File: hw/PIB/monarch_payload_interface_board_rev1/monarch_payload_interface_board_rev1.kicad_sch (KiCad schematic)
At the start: 0 parts

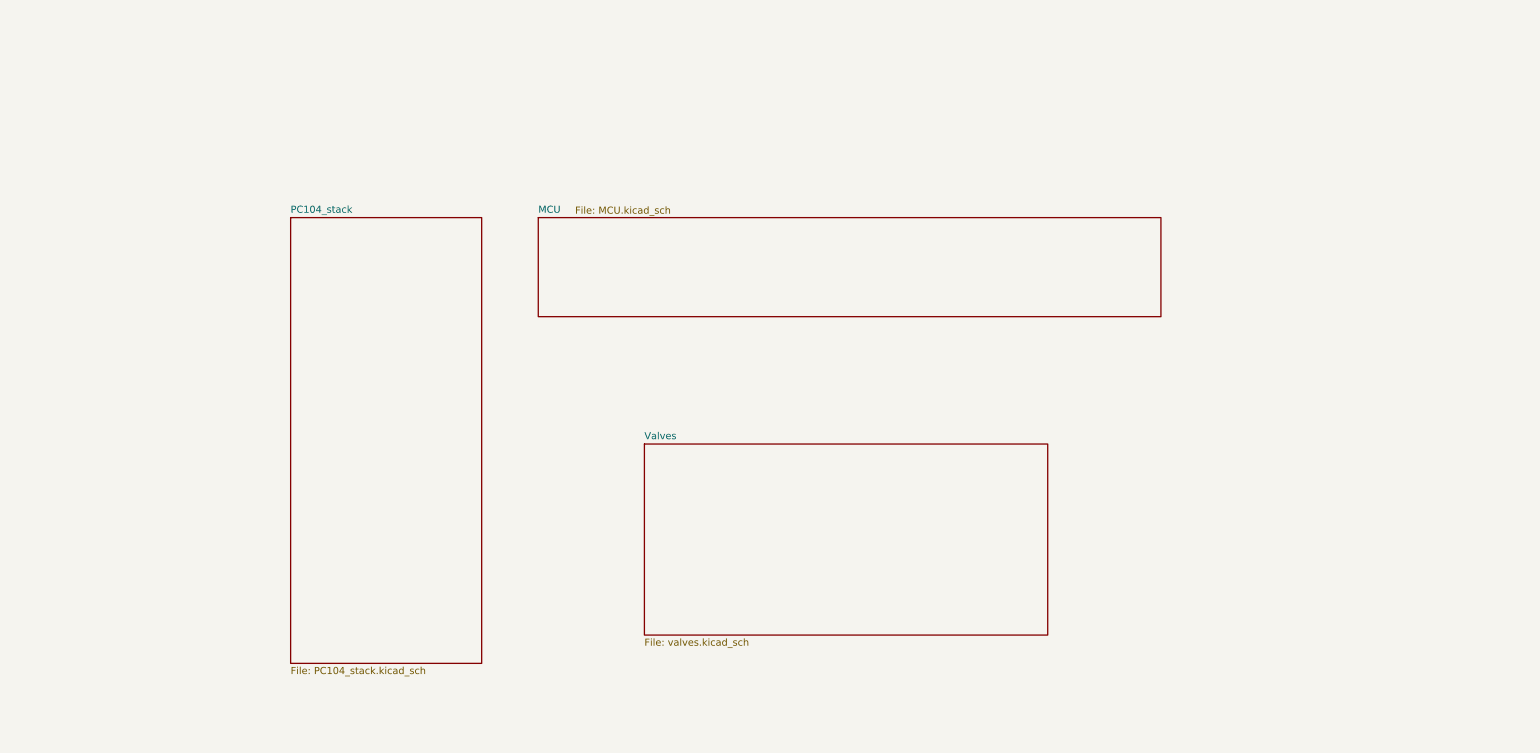
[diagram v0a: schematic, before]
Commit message: More components
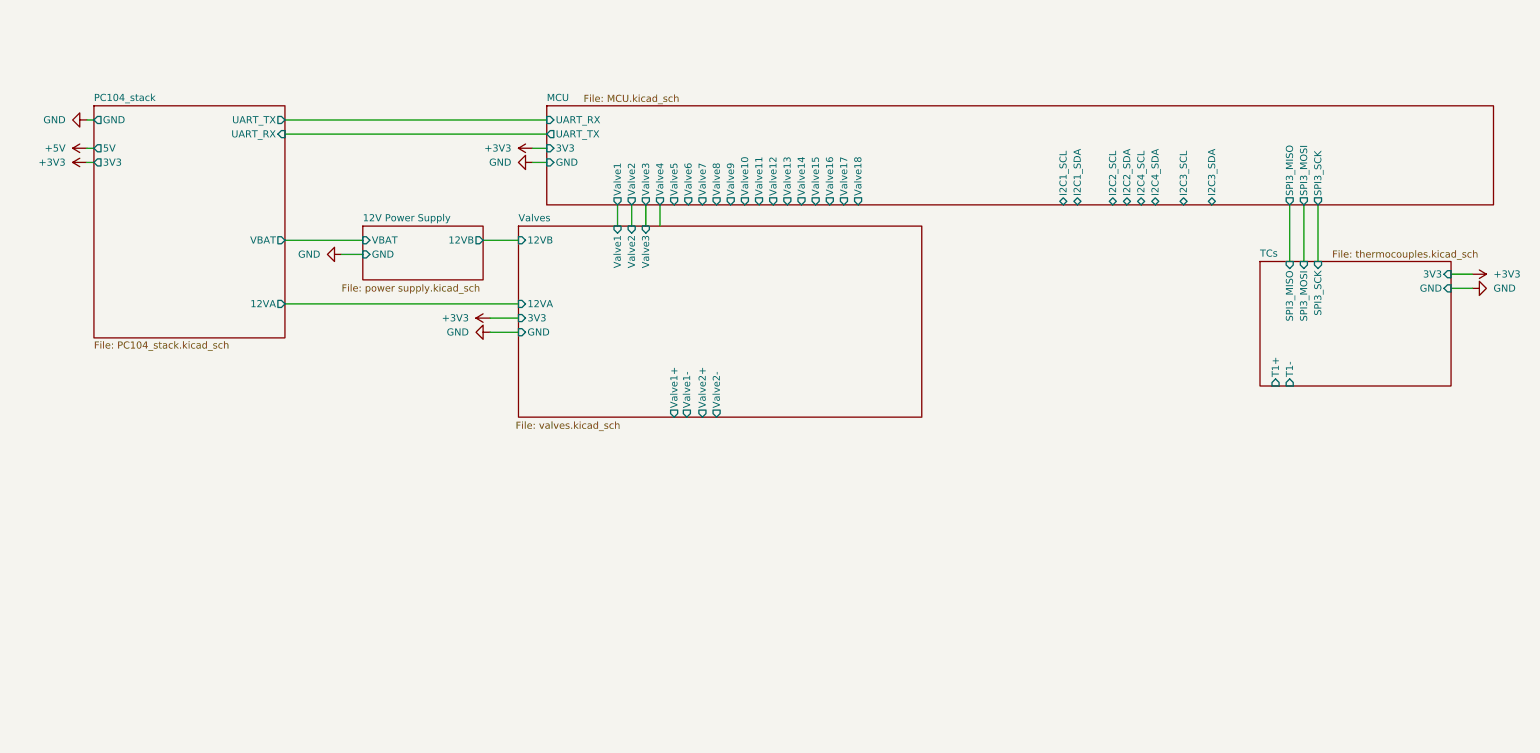
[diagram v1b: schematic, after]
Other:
- added sheet 12V Power Supply (power supply.kicad_sch)
- added sheet TCs (thermocouples.kicad_sch)
- sheet MCU ports: added 3V3, GND, I2C1_SCL, I2C1_SDA, I2C2_SCL, I2C2_SDA, I2C3_SCL, I2C3_SDA, I2C4_SCL, I2C4_SDA, SPI3_MISO, SPI3_MOSI, SPI3_SCK, UART_RX, UART_TX, Valve1, Valve10, Valve11, Valve12, Valve13, Valve14, Valve15, Valve16, Valve17, Valve18, Valve2, Valve3, Valve4, Valve5, Valve6, Valve7, Valve8, Valve9; removed none
- sheet PC104_stack ports: added 12VA, 3V3, 5V, GND, UART_RX, UART_TX, VBAT; removed none
- sheet Valves ports: added 12VA, 12VB, 3V3, GND, Valve1, Valve1+, Valve1-, Valve2, Valve2+, Valve2-, Valve3; removed none

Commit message: Schematic Review
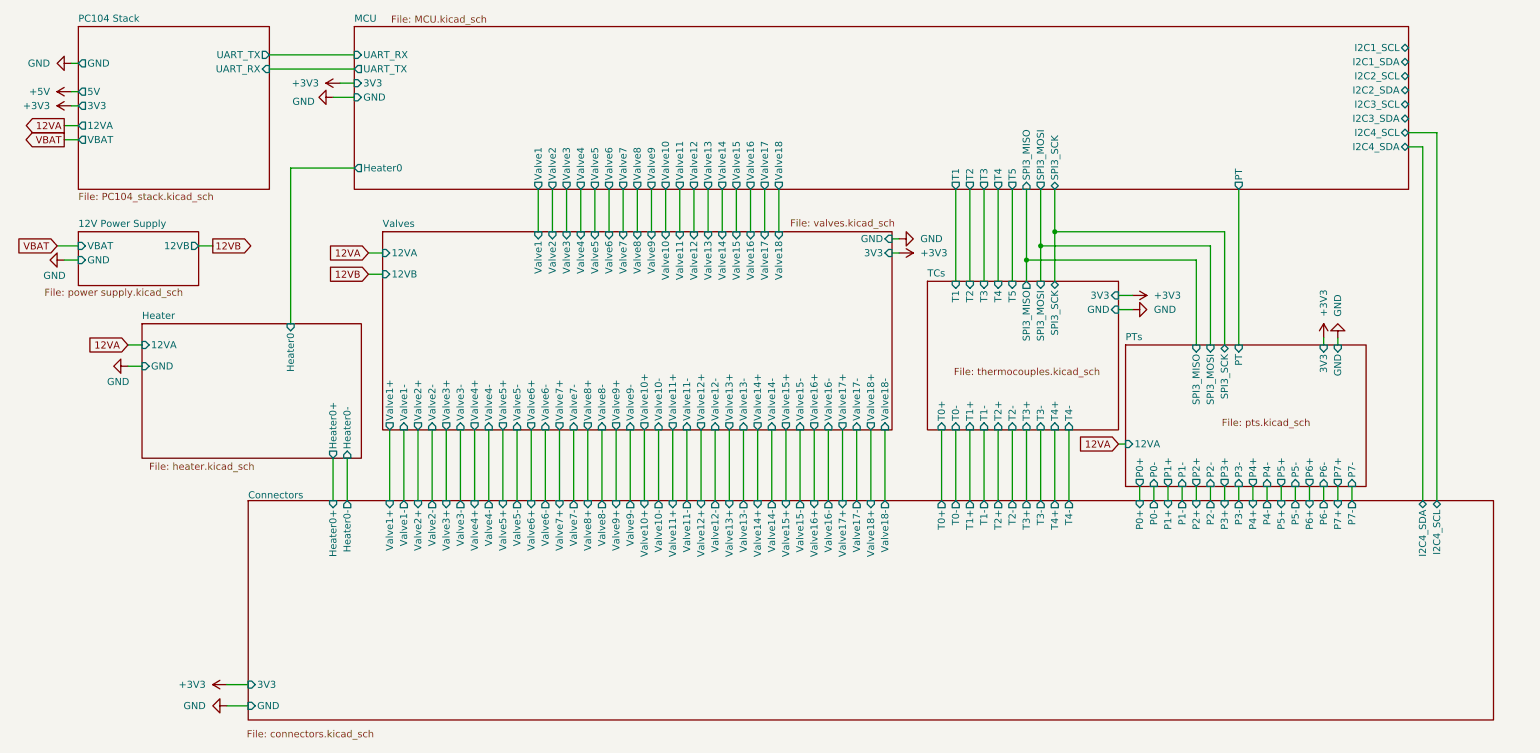
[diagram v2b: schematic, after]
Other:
- sheet PC104_stack renamed PC104 Stack
- added sheet Connectors (connectors.kicad_sch)
- added sheet Heater (heater.kicad_sch)
- added sheet PTs (pts.kicad_sch)
- sheet MCU ports: added Heater0, PT, T1, T2, T3, T4, T5; removed none
- sheet TCs ports: added T0+, T0-, T1, T2, T2+, T2-, T3, T3+, T3-, T4, T4+, T4-, T5; removed none
- sheet Valves ports: added Valve10, Valve10+, Valve10-, Valve11, Valve11+, Valve11-, Valve12, Valve12+, Valve12-, Valve13, Valve13+, Valve13-, Valve14, Valve14+, Valve14-, Valve15, Valve15+, Valve15-, Valve16, Valve16+, Valve16-, Valve17, Valve17+, Valve17-, Valve18, Valve18+, Valve18-, Valve3+, Valve3-, Valve4, Valve4+, Valve4-, Valve5, Valve5+, Valve5-, Valve6, Valve6+, Valve6-, Valve7, Valve7+, Valve7-, Valve8, Valve8+, Valve8-, Valve9, Valve9+, Valve9-; removed none
